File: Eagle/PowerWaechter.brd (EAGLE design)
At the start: 100 x 80 mm, 13 parts, among them U1 ESP32-DEVKITC-32D, X1 12V, X2 JST-XH-03-PIN-ROUND-PAD, X3 JST-XH-03-PIN-ROUND-PAD, X4 Versorgung, X5 230V | N | L

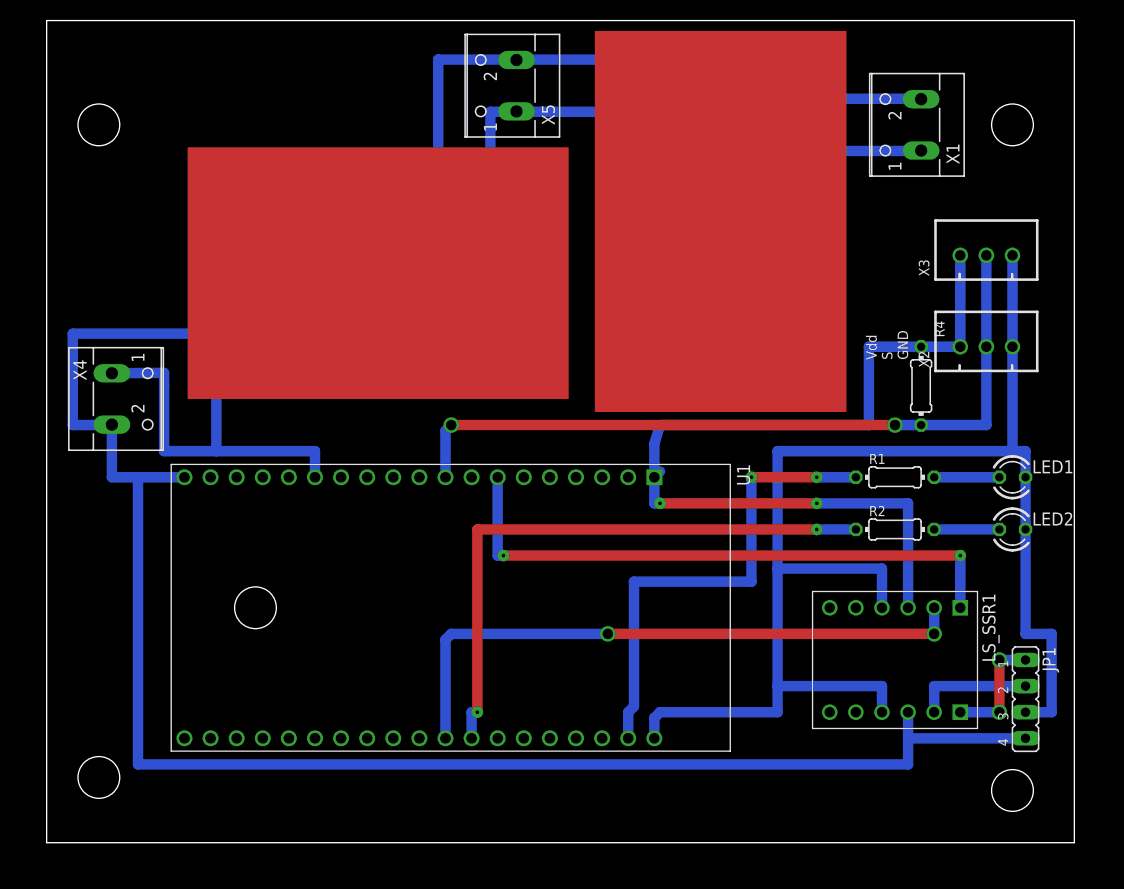
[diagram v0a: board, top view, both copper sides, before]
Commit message: v2.0.0 überführt
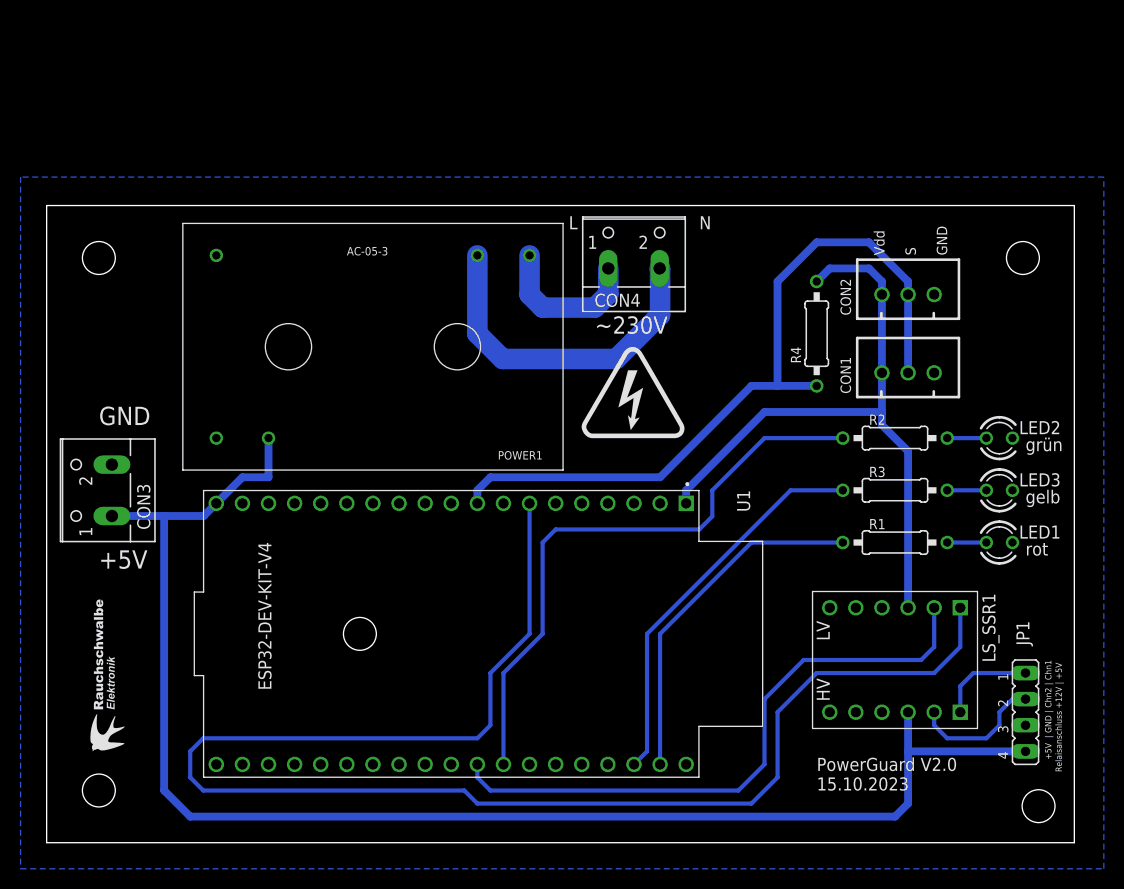
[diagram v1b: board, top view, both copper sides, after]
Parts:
- removed X1: 12V, con-wago-500:W237-102
- removed X2, X3: JST-XH-03-PIN-ROUND-PAD, Rembrandt Electronics - JST XH Connectors v1-0:JST-XH-03-PACKAGE-ROUND-PAD
- removed X4: Versorgung, con-wago-500:W237-102
- removed X5: 230V | N | L, con-wago-500:W237-102
- added CON1, CON2: JST-XH-03, PowerGuard:JST-XH-03
- added CON3, CON4: (no value), PowerGuard:WAGO-500-2
- added LED3: gelb, PowerGuard:LED3MM
- added POWER1: AC-05-3, PowerGuard:AC-05-3
- added R3: 220, PowerGuard:0207/10
- added U$1: WARNLABLE_BLITZ_KLEIN, PowerGuard:WARNLABLE_BLITZ_KLEIN
- added U$2: LOGO_RAUCHSCHWALBE_KLEIN, PowerGuard:LOGO_RAUCHSCHWALBE_KLEIN
- LED1: value red -> rot; device led:LED3MM -> PowerGuard:LED3MM
- LED2: device led:LED3MM -> PowerGuard:LED3MM
- LS_SSR1: value BOB-12009 -> LEVELSHIFTER; device BOB-12009:CONV_BOB-12009 -> PowerGuard:LEVELSHIFTER
- R1, R4: device rcl:0204/7 -> PowerGuard:0207/10
- R2: value 220 -> 330; device rcl:0204/7 -> PowerGuard:0207/10
- U1: value ESP32-DEVKITC-32D -> ESP32-DEV-KIT-V4; device ESP32-DEVKITC-32D:MODULE_ESP32-DEVKITC-32D -> PowerGuard:ESP32-DEV-KIT-V4
- moved R4 11.4 mm to (74.9, 49.5)
- moved LED2 8.98 mm to (92.7, 39.4)
- moved R2 8.89 mm to (82.5, 39.4)
- moved LED1 6.48 mm to (92.7, 29.2)
- moved R1 6.35 mm to (82.5, 29.2)
- moved U1 2.54 mm to (39.4, 20.3)
- moved JP1 1.27 mm to (95.2, 12.7)
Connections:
- removed net GND$2: JP1.3, LED1.K, LED2.K, LS_SSR1.GND_1, LS_SSR1.GND_2, U1.14, U1.20, U1.26, X2.3, X3.3, X4.1
- removed net N$13: U1.6
- removed net N$22: U1.3
- removed net N$3: U1.5
- removed net VDD3$13: LS_SSR1.LV, R4.1, U1.1, X2.1, X3.1
- removed net VDD5$3: JP1.4, LS_SSR1.HV, U1.19, X4.2
- new net +3V3: CON1.1, CON2.1, LS_SSR1.LV, R4.1, U1.1
- new net +5V: CON3.1, JP1.4, LS_SSR1.HV, POWER1.5, U1.19
- new net GND: CON1.3, CON2.3, CON3.2, JP1.3, LED1.K, LED2.K, LED3.K, LS_SSR1.GND_1, LS_SSR1.GND_2, POWER1.4, U1.14, U1.32, U1.38
- new net N$5: LED3.A, R3.2
- new net N$9: R3.1, U1.36
- new net PHASE_L: CON4.1, POWER1.1
- new net PHASE_N: CON4.2, POWER1.2
- net N$1: now also U1.37; no longer U1.21
- net N$11: now also CON1.2, CON2.2; no longer X2.2, X3.2
- net N$16: now also U1.30; no longer U1.28
- net N$6: now also U1.31; no longer U1.27
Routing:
- net GND$2: track 178.7 -> 0.00 mm
- net VDD5$3: track 165.9 -> 0.00 mm
- net +5V: track 0.00 -> 141.6 mm
- net VDD3$13: track 89.1 -> 0.00 mm, vias 2 -> 0
- net N$10: track 57.7 -> 145.8 mm, vias 2 -> 0
- net +3V3: track 0.00 -> 63.7 mm
- net N$14: track 45.7 -> 0.00 mm
- net PHASE_N: track 0.00 -> 32.7 mm
- net N$5: track 30.5 -> 3.81 mm
- net N$12: track 19.0 -> 0.00 mm
- net PHASE_L: track 0.00 -> 15.0 mm
- net N$1: track 47.2 -> 34.2 mm, vias 2 -> 0
- net N$9: track 47.0 -> 38.1 mm
- net N$8: track 6.35 -> 3.81 mm
- net N$7: track 6.35 -> 3.81 mm
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- added copper zone on layer 16, net GND
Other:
- board size 100 x 80 mm -> 100 x 62 mm
- board text added: "L"
- board text added: "N"
- board text added: "PowerGuard V2.0 15.10.2023"
- board text added: "Relaisanschluss +12V | +5V"
- board text added: "gelb"
- board text added: "grün"
- board text added: "rot"
- board text added: "~230V"
- board text removed: "AC-12-3"
